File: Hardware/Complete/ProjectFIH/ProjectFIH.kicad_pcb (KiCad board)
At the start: 2 copper layers, 94 x 99.1 mm, 84 parts, among them J1 Conn_01x02_Male, J10 Payload LED, J2 Power, J3 Power LED, J4 MCU Fail LED, J5 Heater LED, J6 Heater, J7 UART, J8 AVR-ISP-10, J9 Payload, Q1 2N7002, Q2 2N7002, Q3 IRLZ44N, U1 74HC04, U2 74HC08, U3 74HC02, U4 LM158, U5 74HC4017, U6 LM22675-5.0, U7 LM2576S-ADJ, U8 ATmega8A-AU, Y1 8MHz

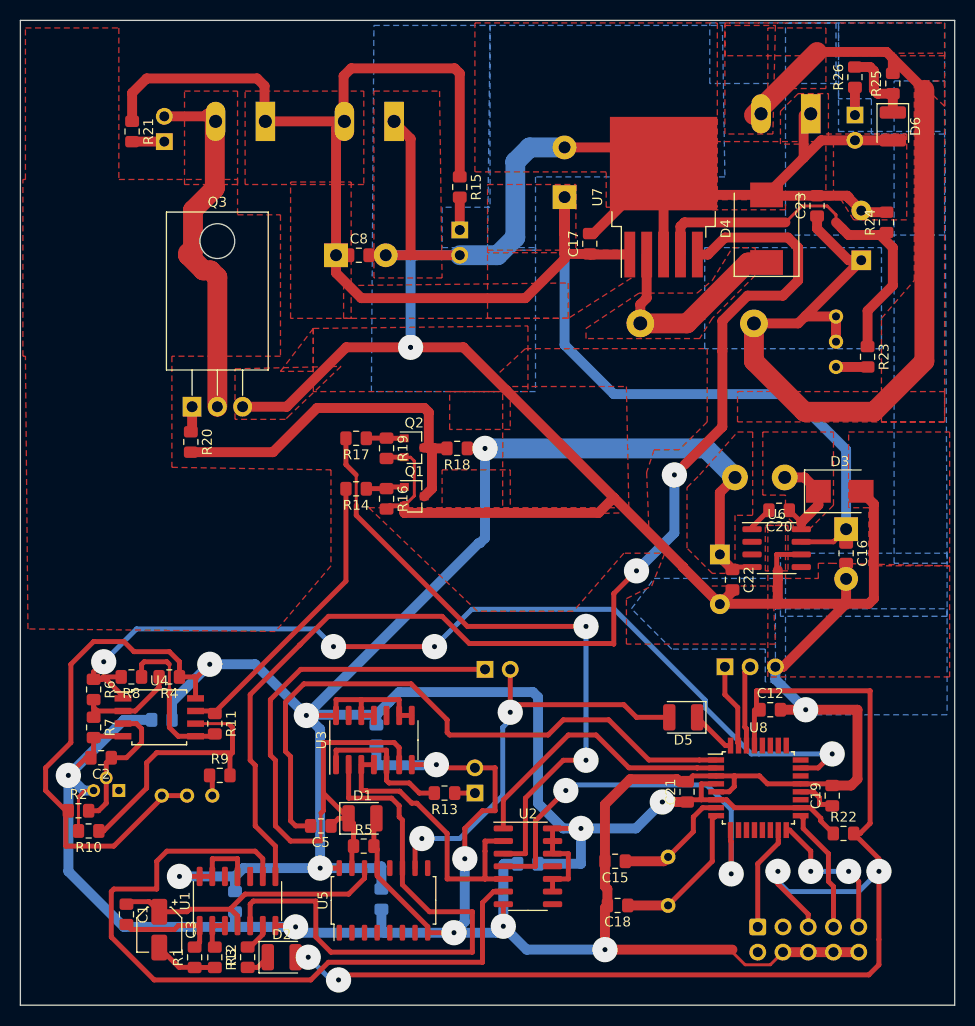
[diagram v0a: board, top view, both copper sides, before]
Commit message: Most of metallization
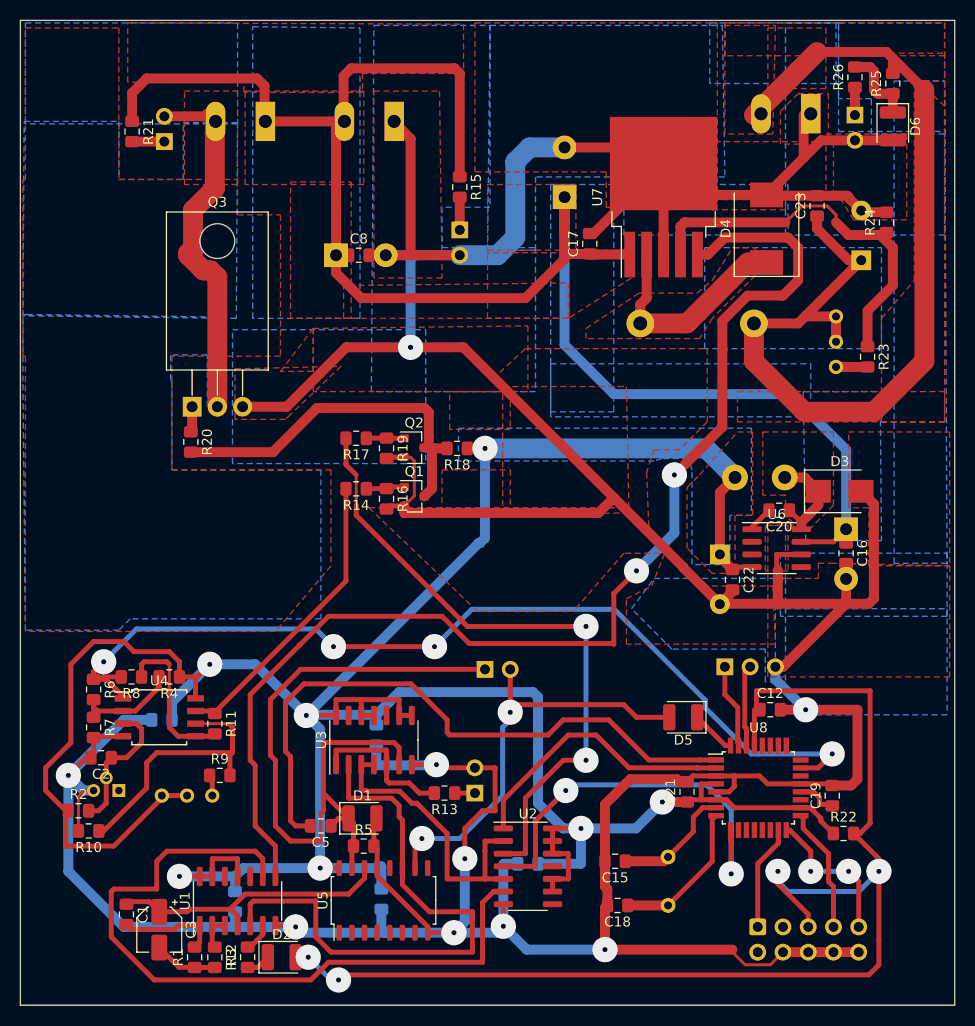
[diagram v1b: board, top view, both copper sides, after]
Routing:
- added copper zone on B.Cu, net +24V
- added copper zone on B.Cu, net +5V
- added copper zone on B.Cu, net Net-(J5-Pad2)
